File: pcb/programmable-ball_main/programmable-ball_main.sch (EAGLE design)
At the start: 30 parts, among them J1 12402012E212A, J3 B4B-ZR-SM4-TFT(LF)(SN), P1 S2B-ZR-SM4A-TF, Q1 DMG2305UX-13, U1 MDBT50Q-1MV2, U2 AP2112K-3.3TRG1, U3 MCP73832T-2ACI/OT, Y1 FC-135_32.7680KA-A0

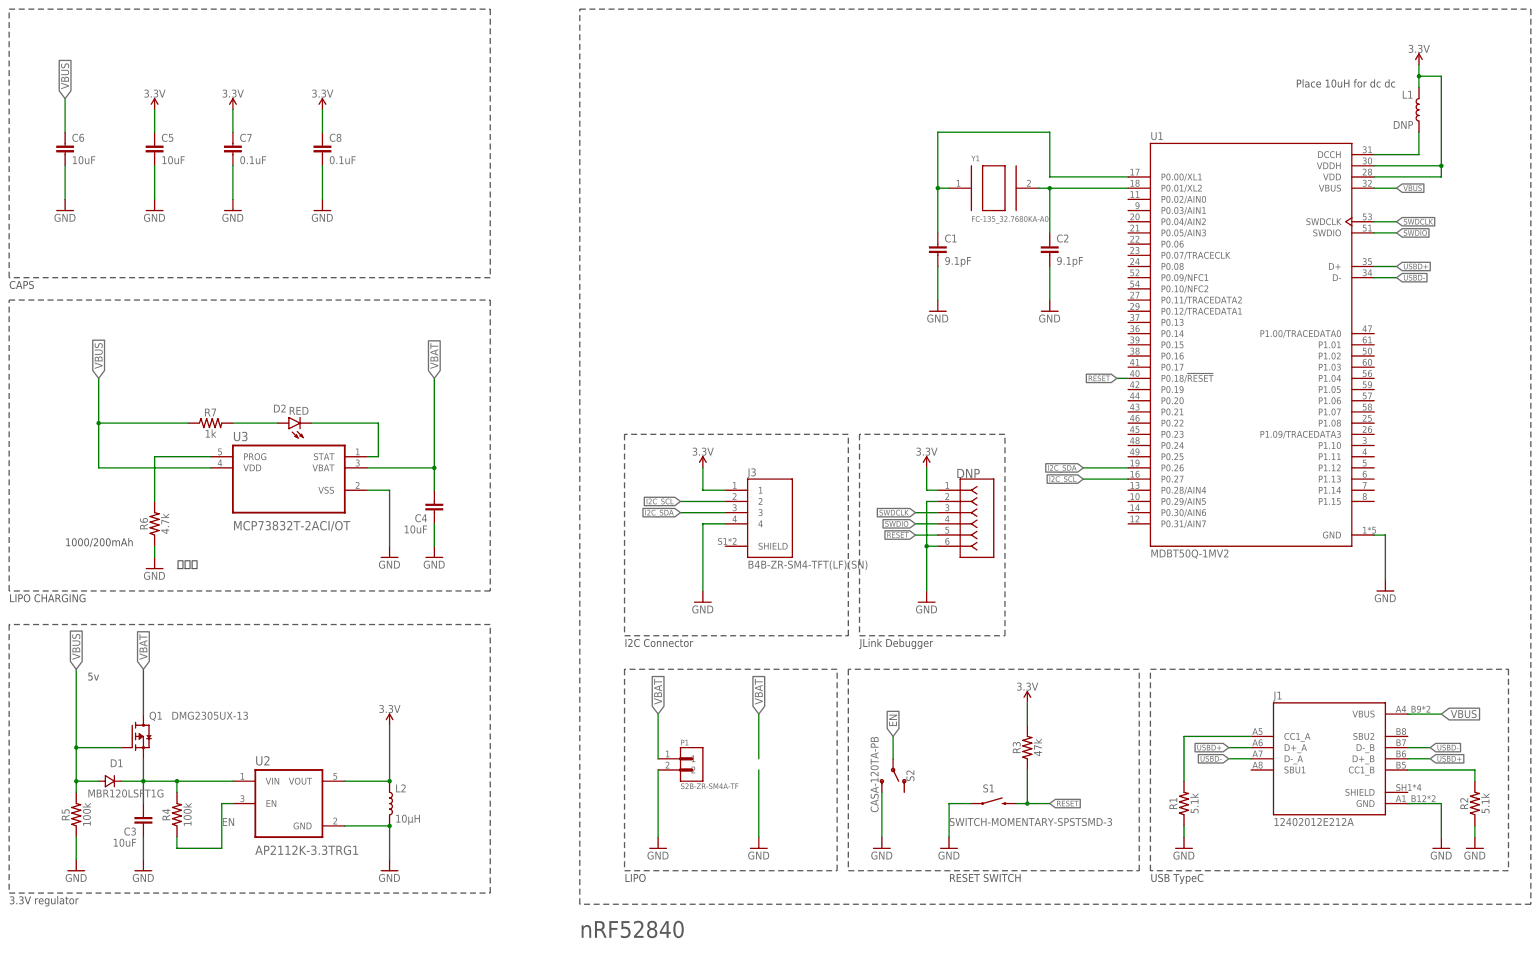
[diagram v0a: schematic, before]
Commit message: v1の修正
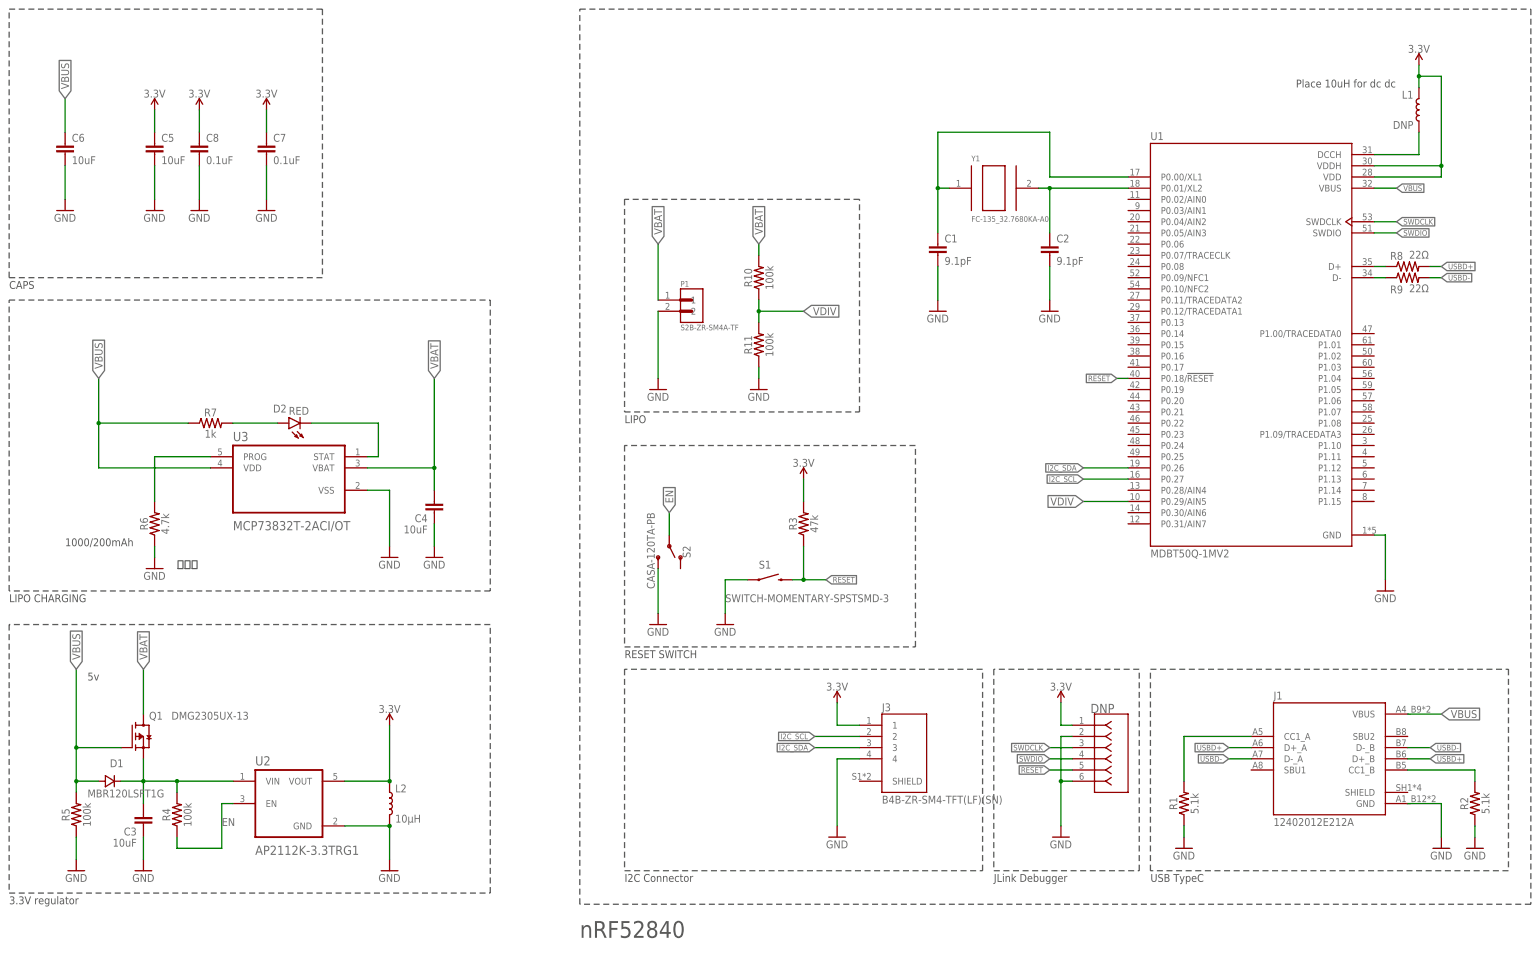
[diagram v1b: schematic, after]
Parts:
- added R10, R11: 100k, SparkFun-Resistors:100KOHM-0402T-1/16W-1%
- added R8, R9: 22Ω, SparkFun-Resistors:22OHM-0402T-1/16W-1%
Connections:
- new net N$10: R8.1, U1.D+
- new net N$11: R9.1, U1.D-
- new net VDIV: R10.1, R11.2, U1.P0.29/AIN5
- net GND: now also R11.1
- net USBD+: now also R8.2; no longer U1.D+
- net USBD-: now also R9.2; no longer U1.D-
- net VBAT: now also R10.2
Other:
- moved on the sheet: C7, C8, DNP, J3, P1, R3, S1, S2
